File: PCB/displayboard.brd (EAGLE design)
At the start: 19.7 x 23.9 mm, 9 parts, among them J1 FTSH-105-01-L-DV

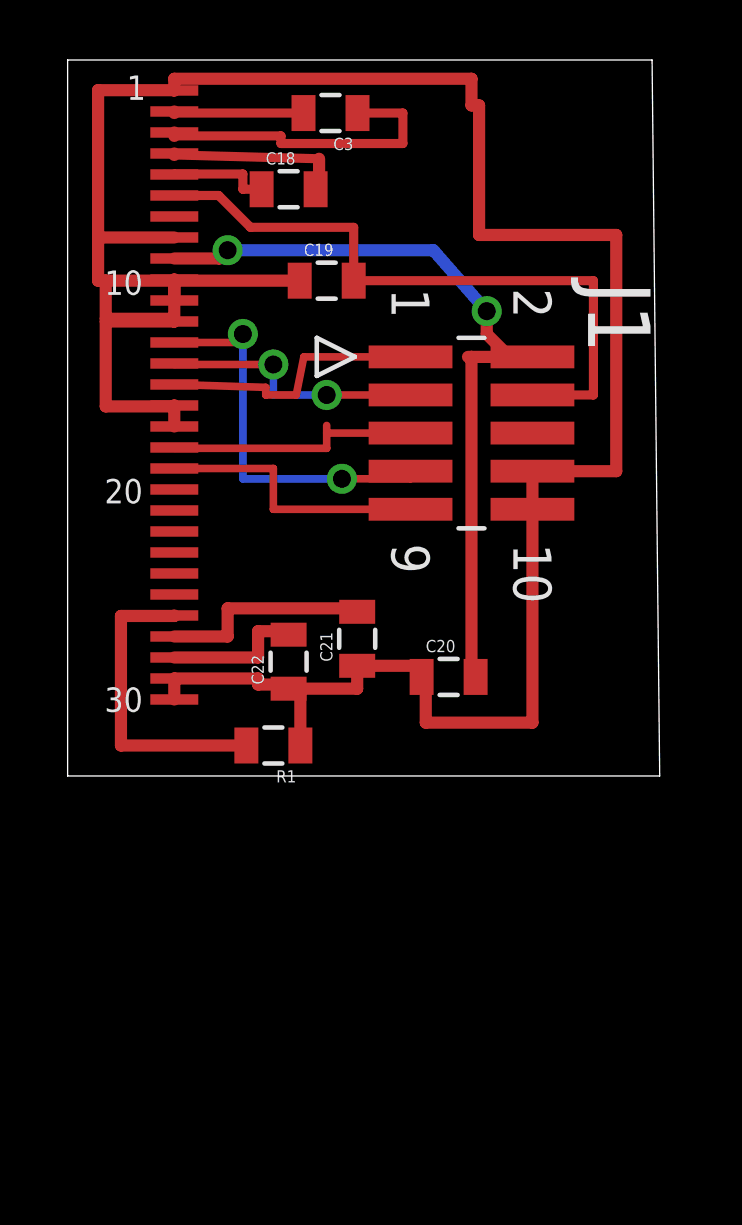
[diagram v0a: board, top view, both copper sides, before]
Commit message: Final version of both PCBs.. Send to OSHPark
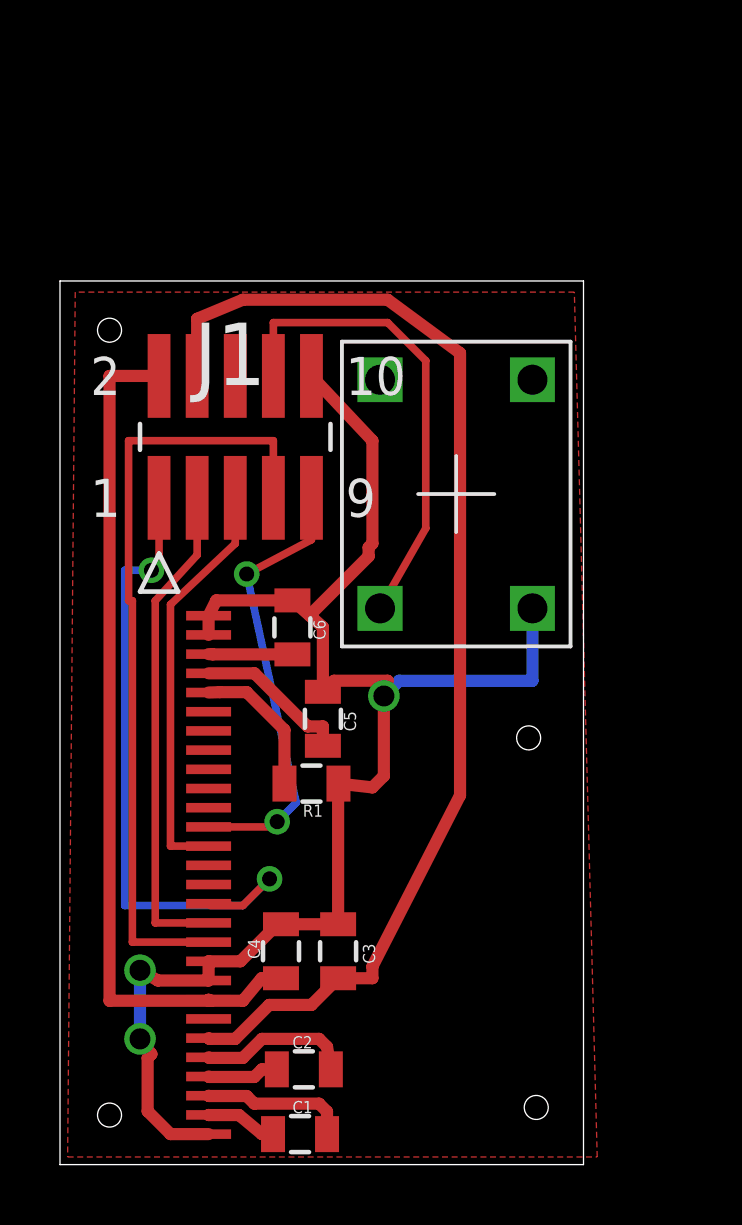
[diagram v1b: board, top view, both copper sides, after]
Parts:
- removed C18: (no value), SparkFun-Capacitors:0805
- removed C19, C20: 2.2u, SparkFun-Capacitors:0805
- removed C21: 4.7uF, SparkFun-Capacitors:0805
- removed C22: 10uF, SparkFun-Capacitors:0805
- added C1, C2: 1uF, SparkFun-Capacitors:0805
- added C4: 2.2u, SparkFun-Capacitors:0805
- added C5: 4.7uF, SparkFun-Capacitors:0805
- added C6: 10uF, SparkFun-Capacitors:0805
- added DISP_SW: (no value), SparkFun-Electromechanical:KSA_SEALED_TAC_SWITCH
- C3: value (none) -> 2.2u
- U$1: device adafruit:1X30-0.7MM -> adafruit:1X28-0.32MM
- moved C3 27.9 mm to (9.27, 6.86), turned to 270 degrees
- moved U$1 24.7 mm to (4.95, 0.76), turned to 90 degrees
- moved J1 7.88 mm to (5.84, 24.0), turned to 0 degrees
- moved R1 1.80 mm to (8.38, 12.4)
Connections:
- new net DISP_SW: DISP_SW.P$1, J1.8
- net 3.3V: now also C4.2, U$1.P$8; no longer C20.2, U$1.9
- net DISP_CS: now also U$1.P$11; no longer U$1.13
- net DISP_DC: now also U$1.P$13; no longer U$1.15
- net GND: now also C3.1, C4.1, C5.1, C6.1, DISP_SW.P$3, U$1.P$1, U$1.P$10, U$1.P$27, U$1.P$28, U$1.P$7, U$1.P$9; no longer C19.1, C20.1, C21.1, C22.1, J1.8, U$1.1, U$1.10, U$1.11, U$1.12, U$1.16, U$1.17, U$1.29, U$1.30, U$1.8
- net N$2: now also C2.1, U$1.P$5; no longer C18.1, U$1.5
- net N$25: now also C1.2, U$1.P$2; no longer C3.2, U$1.2
- net N$26: now also C6.2, U$1.P$26; no longer C22.2, U$1.28
- net N$27: now also C1.1, U$1.P$3; no longer C3.1, U$1.3
- net N$28: now also C5.2, U$1.P$25; no longer C21.2, U$1.27
- net N$29: now also C2.2, U$1.P$4; no longer C18.2, U$1.4
- net N$3: now also U$1.P$24; no longer U$1.26
- net RST: now also U$1.P$12; no longer U$1.14
- net SPI0_MOSI: now also U$1.P$17; no longer U$1.19
- net SPI0_SCK: now also U$1.P$16; no longer U$1.18
- net VBAT: now also C3.2, U$1.P$6; no longer C19.2, U$1.6
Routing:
- net GND: track 89.3 -> 51.5 mm, vias 0 -> 3
- net VBAT: track 22.0 -> 39.2 mm
- net DISP_SW: track 0.00 -> 16.0 mm
- net DISP_DC: track 9.17 -> 22.4 mm, vias 0 -> 2
- net DISP_CS: track 13.2 -> 26.1 mm, vias 2 -> 0
- net RST: track 8.92 -> 16.5 mm, vias 2 -> 0
- net SPI0_MOSI: track 9.23 -> 14.9 mm, vias 0 -> 2
- net N$27: track 10.5 -> 4.92 mm
- net N$3: track 10.3 -> 4.84 mm
- net SPI0_SCK: track 8.66 -> 13.8 mm
- net N$29: track 5.92 -> 2.39 mm
- net 3.3V: track 26.2 -> 28.6 mm, vias 2 -> 0
- net N$26: track 4.80 -> 2.79 mm
- net N$25: track 4.36 -> 2.38 mm
- net N$28: track 7.15 -> 5.19 mm
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- added copper zone on layer 1, net GND
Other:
- board size 19.7 x 23.9 mm -> 17.4 x 29.5 mm
- board text added: "SwiMate Display Board 1.0 P. Bartell Spring 2014"
